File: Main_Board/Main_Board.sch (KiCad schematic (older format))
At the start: 9 parts

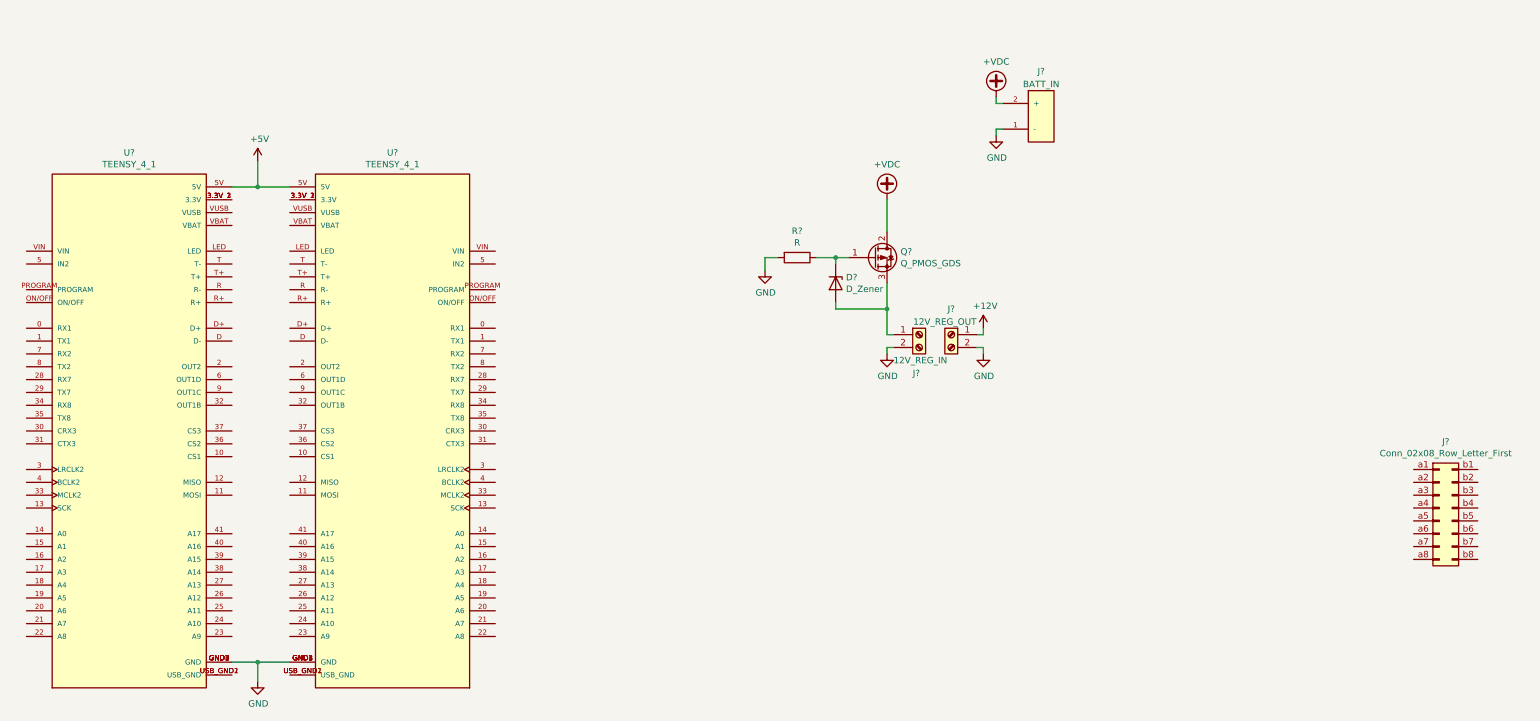
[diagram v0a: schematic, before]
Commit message: Rounding up main and light board
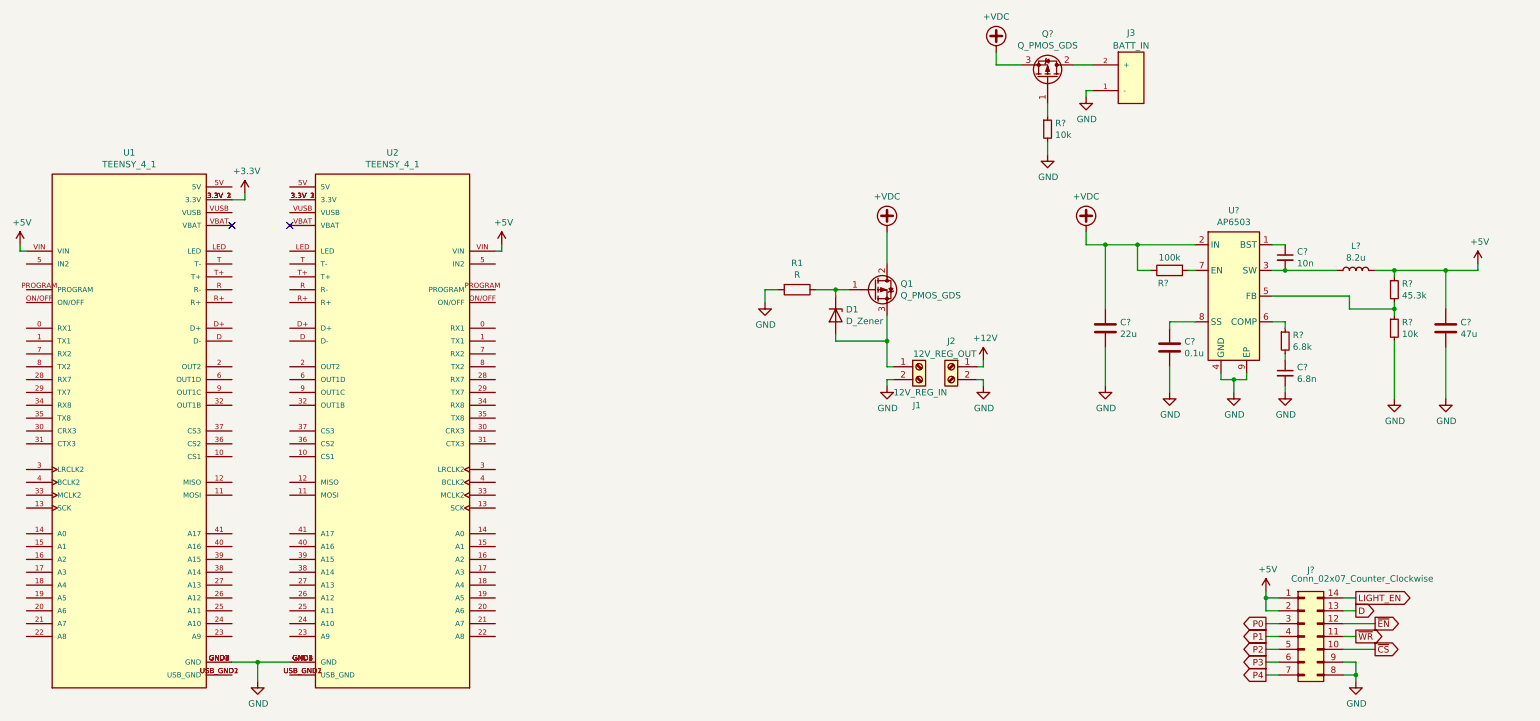
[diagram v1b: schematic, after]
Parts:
- removed J?: Conn_02x08_Row_Letter_First, symbol Connector_Generic:Conn_02x08_Row_Letter_First
- added C?: 0.1u, symbol Device:C
- added C?: 47u, symbol Device:C
- added C?: 10n, symbol Device:C_Small
- added C?: 6.8n, symbol Device:C_Small
- added C?: 22u, symbol Device:C
- added J?: Conn_02x07_Counter_Clockwise, symbol Connector_Generic:Conn_02x07_Counter_Clockwise
- added L?: 8.2u, symbol Device:L
- added Q?: Q_PMOS_GDS, symbol Device:Q_PMOS_GDS
- added R?: 100k, symbol Device:R
- added R?: 45.3k, symbol Device:R_Small
- added R? (x2): 10k, symbol Device:R_Small
- added R?: 6.8k, symbol Device:R_Small
- added U?: AP6503, symbol Regulator_Switching:AP6503
- J3: renamed from J?; footprint AMASS_XT60-M -> (none)
- U1, U2: renamed from U?; footprint MODULE_DEV-16771 -> Main_Board:TEENSY_4_1_FP
- gave numbers to parts that had none: 5
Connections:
- net +5V: now also U1.VIN, U2.VIN, C?.1, J?.1 (Pin_1), J?.2 (Pin_2), L?.2, R?.1; no longer U1.5V, U2.5V
- net +VDC: now also C?.1, Q?.3 (S), R?.1, U?.2 (IN); no longer J3.2 (+)
- net GND: now also C?.2, C?.2, C?.2, C?.2, J?.8 (Pin_8), J?.9 (Pin_9), R?.2, R?.2, U?.4 (GND), U?.9 (EP)
- net +3V3: now reaches U1.3.3V_1 (3.3V), U1.3.3V_2 (3.3V), U1.3.3V_3 (3.3V)
- new net: J3.2 (+), Q?.2 (D)
- new net: C?.1, U?.1 (BST)
- new net: C?.2, L?.1, U?.3 (SW)
- new net: R?.1, R?.2, U?.5 (FB)
- new net: R?.1, U?.6 (COMP)
- new net: R?.2, U?.7 (EN)
- new net: C?.1, U?.8 (SS)
- new net: C?.1, R?.2
- new net: Q?.1 (G), R?.1
- new net D: J?.13 (Pin_13)
- new net LIGHT_EN: J?.14 (Pin_14)
- new net P0: J?.3 (Pin_3)
- new net P1: J?.4 (Pin_4)
- new net P2: J?.5 (Pin_5)
- new net P3: J?.6 (Pin_6)
- new net P4: J?.7 (Pin_7)
- new net ~CS: J?.10 (Pin_10)
- new net ~EN: J?.12 (Pin_12)
- new net ~WR: J?.11 (Pin_11)
- no-connect marks 0 -> 2
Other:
- moved on the sheet: D1, J1, J2, J3, Q1, R1
